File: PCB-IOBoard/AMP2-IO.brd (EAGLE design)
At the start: 100.4 x 80 mm, 37 parts, among them IC3 REG1117, IC4 REG1117

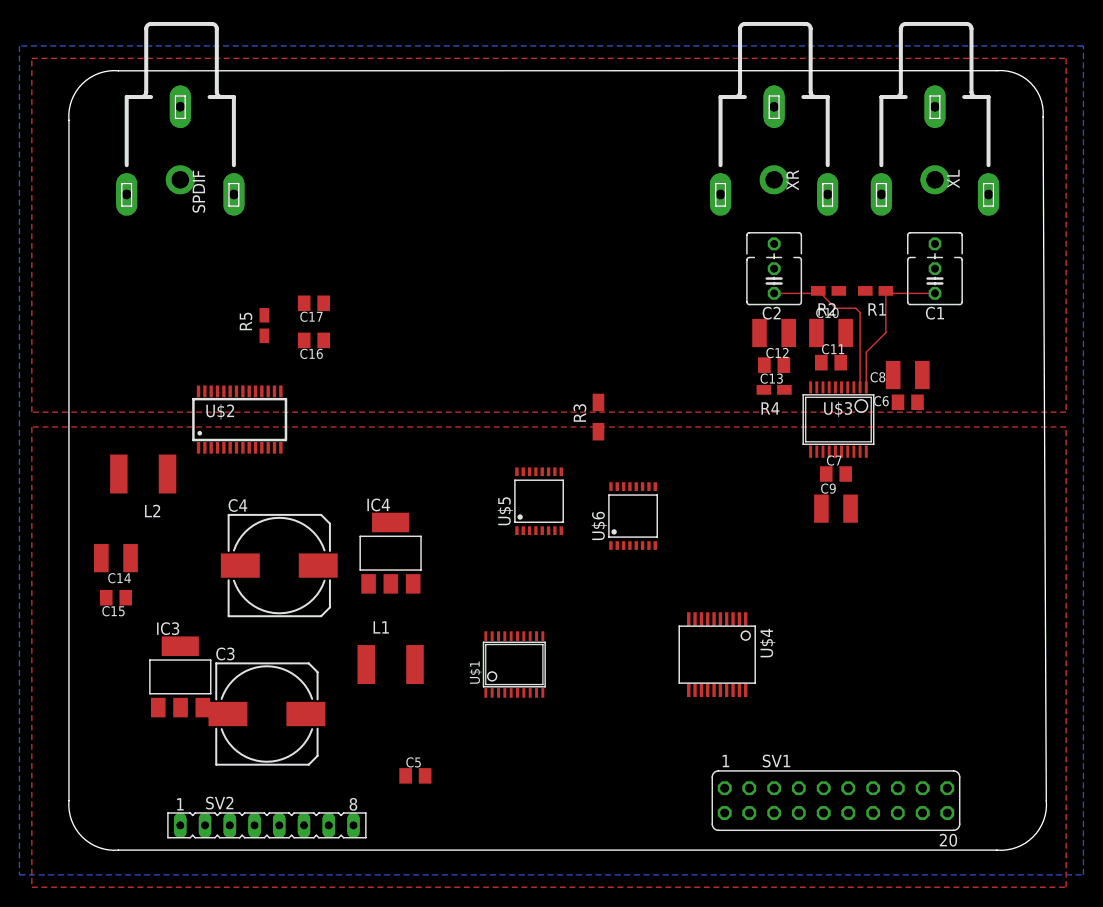
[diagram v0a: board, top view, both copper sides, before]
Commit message: Getting somewhere.
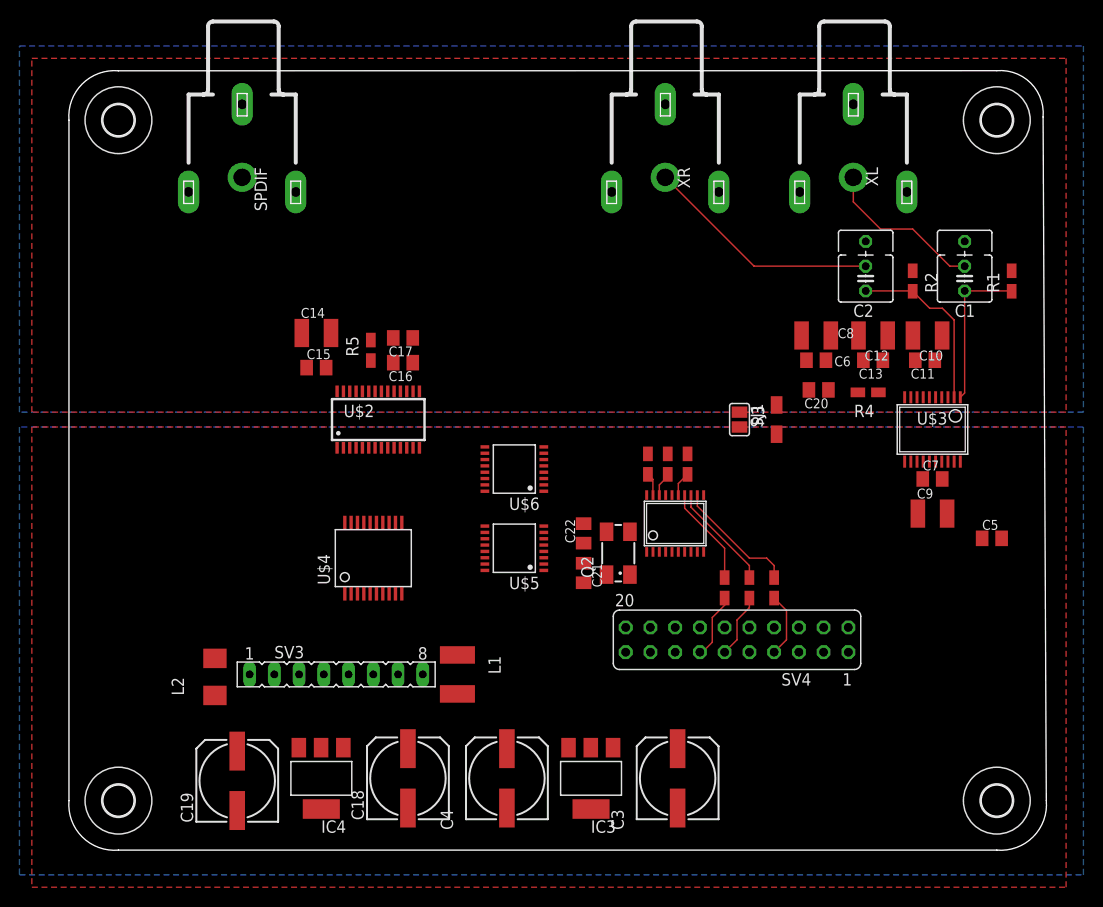
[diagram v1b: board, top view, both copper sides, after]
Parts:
- removed SV1: (no value), con-lsta:FE10-2
- removed SV2: (no value), con-lsta:FE08
- added C18, C19: 100u, rcl:153CLV-0807
- added C20: 100n, rcl:C0805K
- added C21, C22: 12p, rcl:C0805K
- added H1, H2, H3, H4: MOUNT-HOLE3.2, holes:3,2
- added Q2: 12.288, crystal:CTS406
- added R10, R11, R9: 47, rcl:R0805W
- added R6, R8: 4.02k, rcl:R0805W
- added R7: 1k, rcl:R0805W
- added SJ1: (no value), jumper:SJ
- added SV3: (no value), con-lsta:FE08
- added SV4: (no value), con-lsta:FE10-2
- C3, C4: device rcl:153CLV-1010 -> rcl:153CLV-0807
- C5: value (none) -> 100n
- L1: device rcl:L5650M -> rcl:L4532P
- L2: device rcl:L5650M -> rcl:L4532M
- moved C5 64.0 mm to (94.7, 32.0)
- moved IC3 43.4 mm to (53.6, 7.37), turned to 180 degrees
- moved C3 42.7 mm to (62.5, 7.37), turned to 90 degrees
- moved U$4 36.7 mm to (31.2, 30.0), turned to 0 degrees
- moved C4 32.0 mm to (45.0, 7.37), turned to 90 degrees
- moved C15 31.3 mm to (25.4, 49.5), turned to 0 degrees
- moved C14 30.9 mm to (25.4, 53.1), turned to 0 degrees
- moved IC4 24.2 mm to (25.9, 7.37), turned to 180 degrees
- moved L2 22.1 mm to (15.0, 17.8), turned to 90 degrees
- moved U$1 22.0 mm to (62.2, 33.5)
- moved R3 18.3 mm to (72.6, 44.2)
- moved U$2 14.2 mm to (31.8, 44.2)
- moved R1 14.0 mm to (96.8, 58.4), turned to 270 degrees
- moved U$6 13.1 mm to (45.7, 39.1), turned to 90 degrees
- moved R5 11.2 mm to (31.0, 51.3)
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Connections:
- new net +5V: C18.+, IC4.3, SV3.3, SV3.4
- new net ADR/FAULT: SV4.1
- new net GND1: SV3.7, SV3.8
- new net LRCLK: R9.1, SV4.13
- new net MCLK: U$1.10, U$3.15
- new net N$20: C21.2, Q2.1, U$1.2
- new net N$21: R6.1, U$1.15
- new net N$22: R7.1, U$1.19
- new net N$23: R8.1, U$1.18
- new net N$24: C22.2, Q2.3, U$1.1
- new net N$25: R11.2, U$1.12
- new net N$26: R10.2, U$1.13
- new net N$27: R9.2, U$1.14
- new net PDN: SV4.3
- new net SCL: SV4.17, U$4.3
- new net SCLK: R10.1, SV4.11
- new net SDA: SV4.15, U$4.4
- new net SDIN: R11.1, SV4.7
- new net SDOUT: SV4.9
- net +12V: now also SV3.1, SV3.2
- net +3V3: now also C19.+, C5.1, SV3.5, SV3.6, U$3.17, U$3.19, U$3.20, U$3.7
- net A5V: now also C20.1
- net AGND: now also C20.2, SJ1.1
- net GND: now also C18.-, C19.-, C21.1, C22.1, C5.2, R6.2, R7.2, R8.2, SJ1.2, SV4.10, SV4.12, SV4.14, SV4.16, SV4.18, SV4.20, SV4.6, SV4.8, U$3.16, U$3.18, U$3.8
- net SW_BCK: now also U$1.8
- net SW_SCLK: no longer U$1.8
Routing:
- net N$2: track 0.00 -> 24.4 mm
- net N$1: track 0.00 -> 16.7 mm
- net N$25: track 0.00 -> 12.8 mm
- net N$26: track 0.00 -> 11.0 mm
- net N$27: track 0.00 -> 10.2 mm
- net LRCLK: track 0.00 -> 6.75 mm
- net SDIN: track 0.00 -> 6.60 mm
- net SCLK: track 0.00 -> 6.60 mm
- net N$21: track 0.00 -> 2.52 mm
- net N$23: track 0.00 -> 2.48 mm
- net N$22: track 0.00 -> 2.34 mm
- net N$4: track 17.5 -> 18.3 mm
- added copper zone on layer 16, net AGND
